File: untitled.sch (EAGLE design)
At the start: 36 parts, among them J1 61300311121, Q1 FQPF10N60C, Q2 s8550, Q3 s8550, T2 s8050, T3 s8050

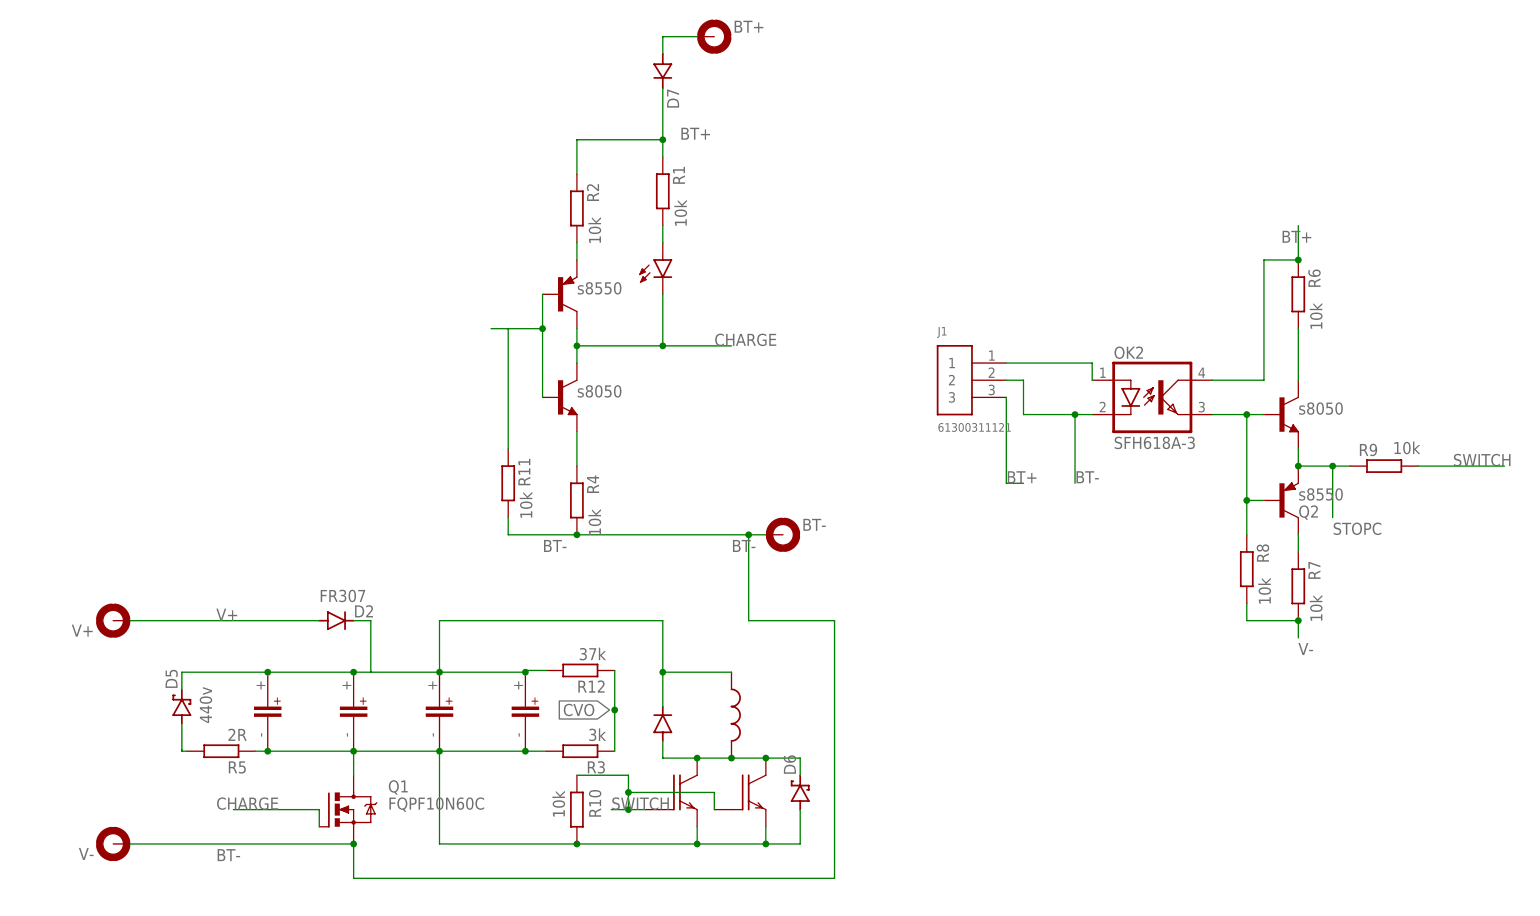
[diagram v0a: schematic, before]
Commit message: add
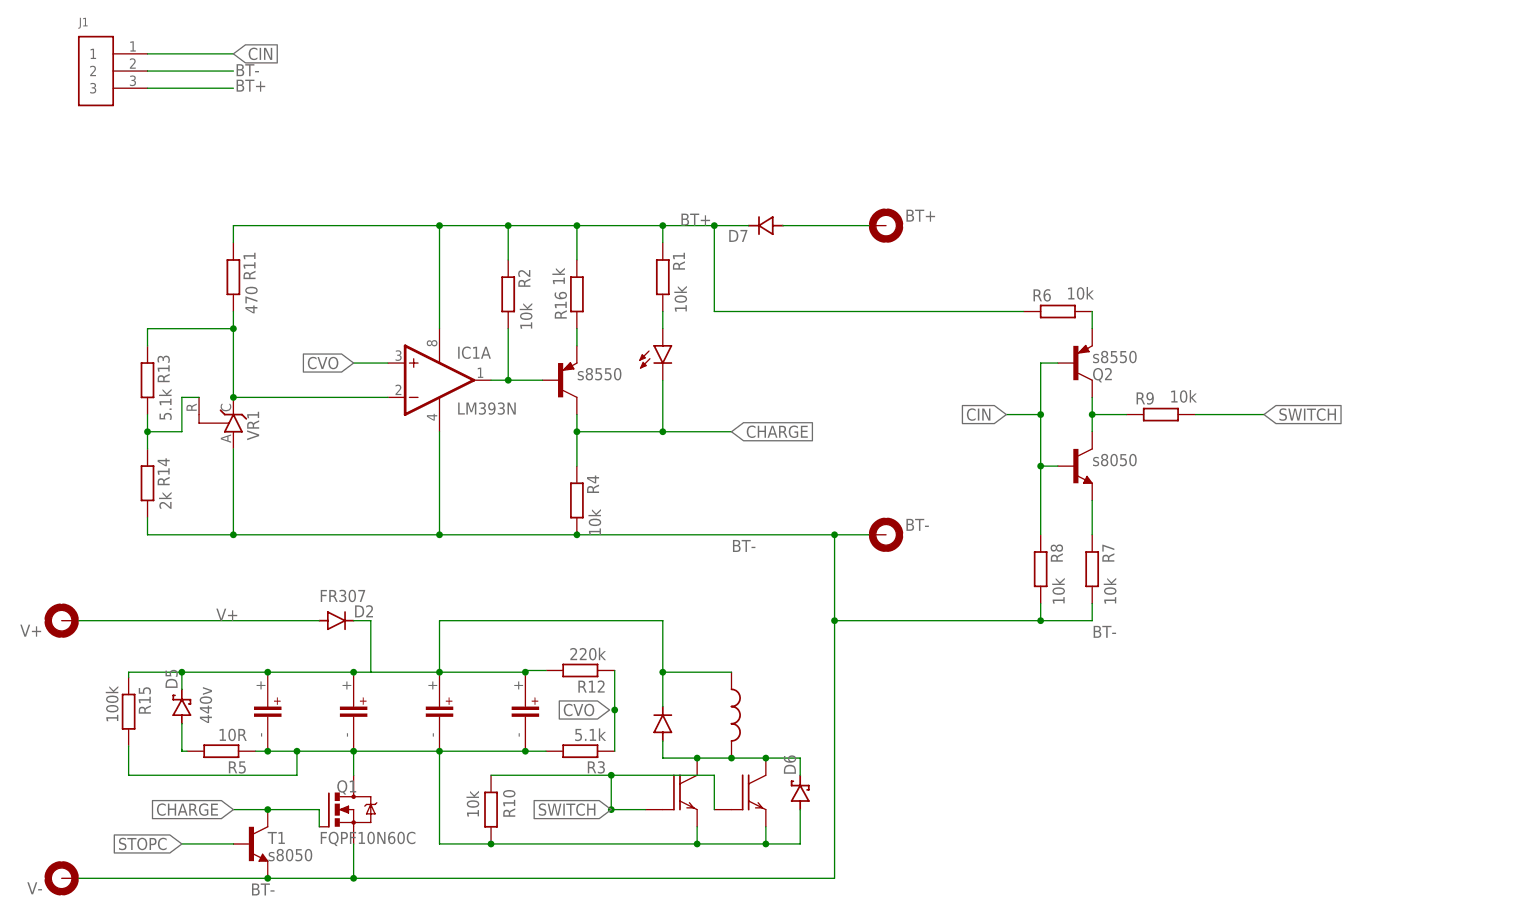
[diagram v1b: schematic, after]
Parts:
- removed OK2: SFH618A-3, optocoupler:SFH618A-3
- removed T2: s8050, transistor:2N3704
- added IC1: LM393N, linear:LM393N
- added R13: 5.1k, rcl:R-EU_0207/2V
- added R14: 2k, rcl:R-EU_0207/2V
- added R15: 100k, rcl:R-EU_0207/2V
- added R16: 1k, rcl:R-EU_0207/2V
- added T1: s8050, transistor:-NPN-TO92
- added VR1: (no value), v-reg:TL431CLP
- R11: value 10k -> 470
- R12: value 37k -> 220k
- R3: value 3k -> 5.1k
- R5: value 2R -> 10R
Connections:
- removed net N$14: R6.2, T3.C
- removed net N$9: Q3.E, R2.2
- removed net V-: R7.2, R8.2
- new net CIN: J1.1, Q2.B, R8.1, T3.B
- new net N$5: IC1A.-IN, R11.2, R13.1, VR1.C
- net BT+: now also IC1P.V+, R11.1, R16.2; no longer OK2.COL
- net BT-: now also IC1P.V-, R14.2, R7.2, R8.2, T1.E, VR1.A; no longer OK2.C, R11.2
- net CHARGE: now also R4.1, T1.C; no longer T2.C
- net CVO: now also IC1A.+IN
- net N$1: now also IC1A.OUT, Q3.B, R2.2; no longer R11.1
- net N$10: now also Q3.E, R16.1; no longer D6.A, Q1.D, R10.1, R3.2, R5.1, U$1.-, U$13.E, U$2.-, U$3.-, U$4.-, U$9.E
- net N$11: now also Q2.E, R6.2; no longer J1.1, OK2.A
- net N$12: now also Q2.C, R9.1, T3.C; no longer OK2.EMIT, Q2.B, R8.1, T3.B
- net N$13: now also T3.E; no longer Q2.C
- net N$7: now also R13.2, R14.1, VR1.R; no longer Q3.B, T2.B
- net N$8: now also D6.A, Q1.D, R10.1, R15.2, R3.2, R5.1, U$1.-, U$13.E, U$2.-, U$3.-, U$4.-, U$9.E; no longer R4.1, T2.E
- net STOPC: now also T1.B; no longer Q2.E, R9.1, T3.E
- net UC: now also R15.1
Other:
- moved on the sheet: BT+, BT-, D7, J1, Q2, R1, R10, R11, R2, R6, R7, R8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

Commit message: add
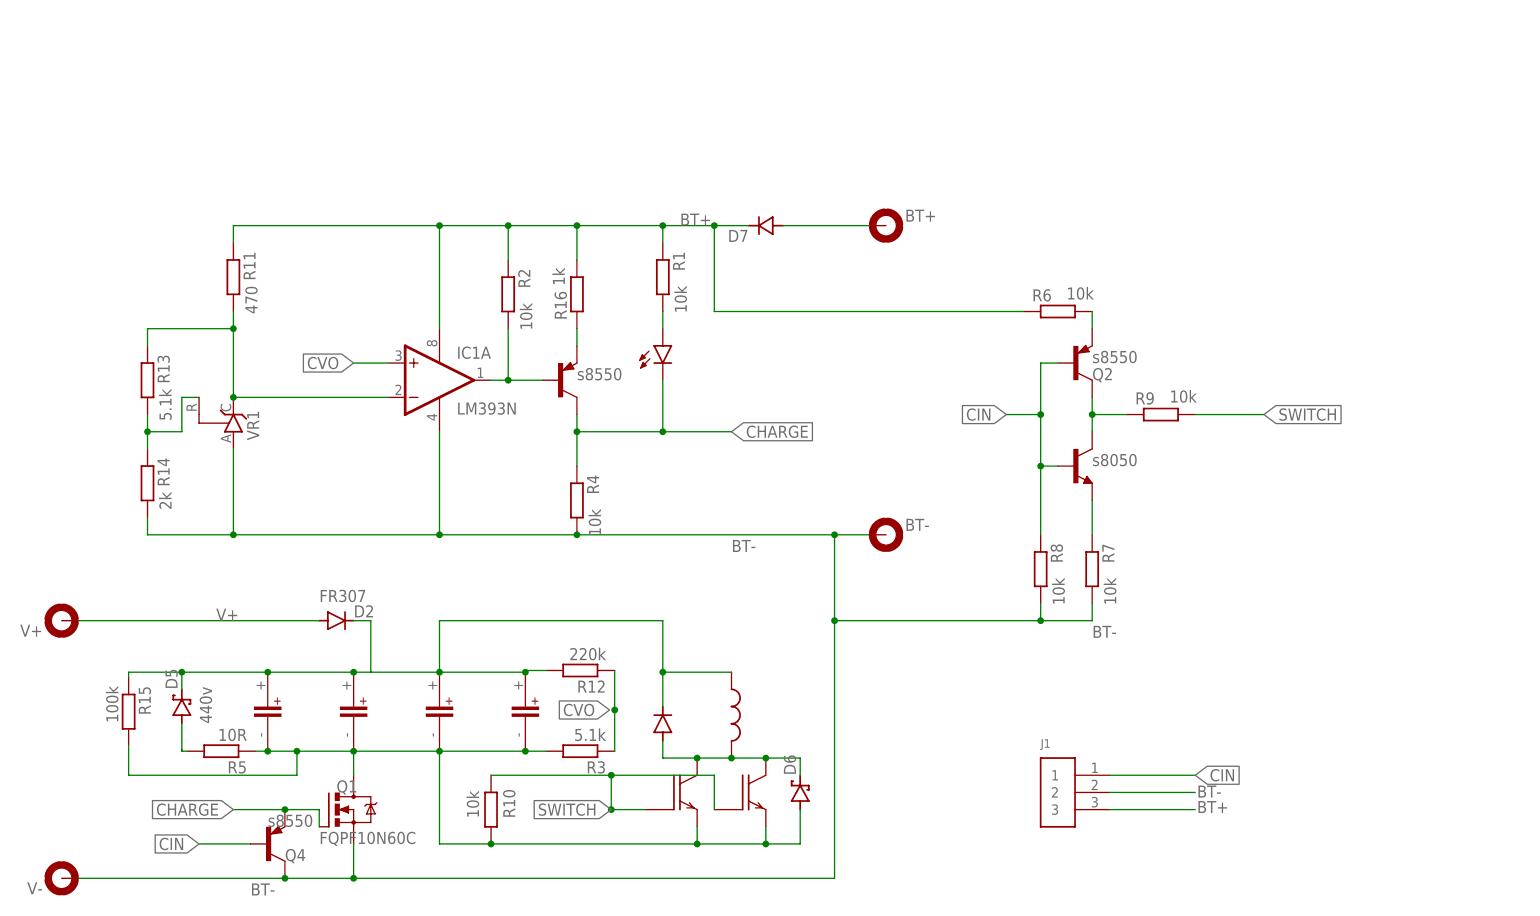
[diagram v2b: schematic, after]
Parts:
- removed T1: s8050, transistor:-NPN-TO92
- added Q4: s8550, transistor-pnp:2N3906
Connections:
- removed net STOPC: T1.B
- net BT-: now also Q4.C; no longer T1.E
- net CHARGE: now also Q4.E; no longer T1.C
- net CIN: now also Q4.B
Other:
- moved on the sheet: J1
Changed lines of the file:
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@@
 <part name="R15" library="rcl" library_urn="urn:adsk.eagle:library:334" deviceset="R-EU_" device="0207/2V" package3d_urn="urn:adsk.eagle:package:23490/1" value="100k"/>
 <part name="R16" library="rcl" library_urn="urn:adsk.eagle:library:334" deviceset="R-EU_" device="0207/2V" package3d_urn="urn:adsk.eagle:package:23490/1" value="1k"/>
-<part name="T1" library="transistor" library_urn="urn:adsk.eagle:library:402" deviceset="*-NPN-" device="TO92" package3d_urn="urn:adsk.eagle:package:28523/2" value="s8050"/>
 <part name="R8" library="rcl" library_urn="urn:adsk.eagle:library:334" deviceset="R-EU_" device="0207/2V" package3d_urn="urn:adsk.eagle:package:23490/1" value="10k"/>
+<part name="Q4" library="transistor-pnp" library_urn="urn:adsk.eagle:library:399" deviceset="2N3906" device="" package3d_urn="urn:adsk.eagle:package:29211/2" value="s8550"/>
 </parts>
 <sheets>
@@
 </instance>
 <instance part="U$13" gate="G$1" x="93.98" y="7.62" smashed="yes"/>
-<instance part="J1" gate="G$1" x="-2.54" y="114.3" smashed="yes">
-<attribute name="NAME" x="-5.08" y="120.904" size="1.27" layer="95"/>
+<instance part="J1" gate="G$1" x="139.7" y="7.62" smashed="yes">
+<attribute name="NAME" x="137.16" y="14.224" size="1.27" layer="95"/>
 </instance>
 <instance part="T3" gate="G$1" x="142.24" y="55.88" smashed="yes">
@@
 <attribute name="VALUE" x="66.802" y="82.55" size="1.778" layer="96" rot="R90"/>
 </instance>
-<instance part="T1" gate="G$1" x="20.32" y="0" smashed="yes">
-<attribute name="NAME" x="22.86" y="0" size="1.778" layer="95"/>
-<attribute name="VALUE" x="22.86" y="-2.54" size="1.778" layer="96"/>
-</instance>
 <instance part="R8" gate="G$1" x="137.16" y="40.64" smashed="yes" rot="R270">
 <attribute name="NAME" x="138.6586" y="44.45" size="1.778" layer="95" rot="R270"/>
 <attribute name="VALUE" x="138.938" y="39.37" size="1.778" layer="96" rot="R270"/>
+</instance>
+<instance part="Q4" gate="G$1" x="22.86" y="0" smashed="yes">
+<attribute name="NAME" x="25.4" y="-2.54" size="1.778" layer="95"/>
+<attribute name="VALUE" x="22.86" y="2.54" size="1.778" layer="96"/>
 </instance>
 </instances>
@@
 <net name="CHARGE" class="0">
 <segment>
-<wire x1="30.48" y1="5.08" x2="22.86" y2="5.08" width="0.1524" layer="91"/>
+<wire x1="30.48" y1="5.08" x2="25.4" y2="5.08" width="0.1524" layer="91"/>
 <pinref part="Q1" gate="G$1" pin="G"/>
-<wire x1="22.86" y1="5.08" x2="17.78" y2="5.08" width="0.1524" layer="91"/>
+<wire x1="25.4" y1="5.08" x2="17.78" y2="5.08" width="0.1524" layer="91"/>
 <wire x1="30.48" y1="5.08" x2="30.48" y2="2.54" width="0.1524" layer="91"/>
 <label x="17.78" y="5.08" size="1.778" layer="95" rot="R180" xref="yes"/>
-<pinref part="T1" gate="G$1" pin="C"/>
-<junction x="22.86" y="5.08"/>
+<pinref part="Q4" gate="G$1" pin="E"/>
+<junction x="25.4" y="5.08"/>
 </segment>
 <segment>
@@
 <pinref part="R1" gate="G$1" pin="2"/>
 <wire x1="81.28" y1="78.74" x2="81.28" y2="76.2" width="0.1524" layer="91"/>
-</segment>
-</net>
-<net name="STOPC" class="0">
-<segment>
-<pinref part="T1" gate="G$1" pin="B"/>
-<wire x1="17.78" y1="0" x2="10.16" y2="0" width="0.1524" layer="91"/>
-<label x="10.16" y="0" size="1.778" layer="95" rot="R180" xref="yes"/>
 </segment>
 </net>
@@
 <segment>
 <pinref part="J1" gate="G$1" pin="3"/>
-<wire x1="5.08" y1="111.76" x2="17.78" y2="111.76" width="0.1524" layer="91"/>
-<label x="18.034" y="111.252" size="1.778" layer="95"/>
+<wire x1="147.32" y1="5.08" x2="160.02" y2="5.08" width="0.1524" layer="91"/>
+<label x="160.274" y="4.572" size="1.778" layer="95"/>
 </segment>
 <segment>
@@
 <segment>
 <pinref part="J1" gate="G$1" pin="1"/>
-<wire x1="5.08" y1="116.84" x2="17.78" y2="116.84" width="0.1524" layer="91"/>
-<label x="17.78" y="116.84" size="1.778" layer="95" xref="yes"/>
+<wire x1="147.32" y1="10.16" x2="160.02" y2="10.16" width="0.1524" layer="91"/>
+<label x="160.02" y="10.16" size="1.778" layer="95" xref="yes"/>
 </segment>
 <segment>
@@
 <junction x="137.16" y="63.5"/>
 </segment>
+<segment>
+<pinref part="Q4" gate="G$1" pin="B"/>
+<wire x1="20.32" y1="0" x2="12.7" y2="0" width="0.1524" layer="91"/>
+<label x="12.7" y="0" size="1.778" layer="95" rot="R180" xref="yes"/>
+</segment>
 </net>
 <net name="BT-" class="0">
 <segment>
 <pinref part="J1" gate="G$1" pin="2"/>
-<wire x1="5.08" y1="114.3" x2="17.78" y2="114.3" width="0.1524" layer="91"/>
-<label x="18.034" y="113.538" size="1.778" layer="95"/>
+<wire x1="147.32" y1="7.62" x2="160.02" y2="7.62" width="0.1524" layer="91"/>
+<label x="160.274" y="6.858" size="1.778" layer="95"/>
 </segment>
 <segment>
@@
 <wire x1="35.56" y1="-5.08" x2="106.68" y2="-5.08" width="0.1524" layer="91"/>
 <pinref part="V-" gate="G$1" pin="MOUNT"/>
-<wire x1="-5.08" y1="-5.08" x2="22.86" y2="-5.08" width="0.1524" layer="91"/>
+<wire x1="-5.08" y1="-5.08" x2="25.4" y2="-5.08" width="0.1524" layer="91"/>
 <junction x="35.56" y="-5.08"/>
 <pinref part="IC1" gate="P" pin="V-"/>
-<wire x1="22.86" y1="-5.08" x2="35.56" y2="-5.08" width="0.1524" layer="91"/>
+<wire x1="25.4" y1="-5.08" x2="35.56" y2="-5.08" width="0.1524" layer="91"/>
 <wire x1="48.26" y1="60.96" x2="48.26" y2="45.72" width="0.1524" layer="91"/>
 <wire x1="48.26" y1="45.72" x2="68.58" y2="45.72" width="0.1524" layer="91"/>
@@
 <wire x1="5.08" y1="45.72" x2="17.78" y2="45.72" width="0.1524" layer="91"/>
 <junction x="17.78" y="45.72"/>
-<pinref part="T1" gate="G$1" pin="E"/>
-<junction x="22.86" y="-5.08"/>
 <wire x1="137.16" y1="33.02" x2="106.68" y2="33.02" width="0.1524" layer="91"/>
 <junction x="137.16" y="33.02"/>
 <junction x="106.68" y="33.02"/>
+<pinref part="Q4" gate="G$1" pin="C"/>
+<junction x="25.4" y="-5.08"/>
 </segment>
 </net>
@@
 </segment>
 </net>
-<net name="N$12" class="0">
-<segment>
-<pinref part="Q2" gate="G$1" pin="C"/>
-<pinref part="T3" gate="G$1" pin="C"/>
-<wire x1="144.78" y1="66.04" x2="144.78" y2="63.5" width="0.1524" layer="91"/>
-<pinref part="R9" gate="G$1" pin="1"/>
-<wire x1="144.78" y1="63.5" x2="144.78" y2="60.96" width="0.1524" layer="91"/>
-<wire x1="149.86" y1="63.5" x2="144.78" y2="63.5" width="0.1524" layer="91"/>
-<junction x="144.78" y="63.5"/>
-</segment>
-</net>
 <net name="N$13" class="0">
 <segment>
@@
 </segment>
 </net>
+<net name="N$9" class="0">
+<segment>
+<pinref part="R9" gate="G$1" pin="1"/>
+<wire x1="149.86" y1="63.5" x2="144.78" y2="63.5" width="0.1524" layer="91"/>
+<pinref part="Q2" gate="G$1" pin="C"/>
+<wire x1="144.78" y1="63.5" x2="144.78" y2="66.04" width="0.1524" layer="91"/>
+<pinref part="T3" gate="G$1" pin="C"/>
+<wire x1="144.78" y1="63.5" x2="144.78" y2="60.96" width="0.1524" layer="91"/>
+<junction x="144.78" y="63.5"/>
+</segment>
+</net>
